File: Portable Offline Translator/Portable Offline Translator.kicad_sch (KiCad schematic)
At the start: 0 parts

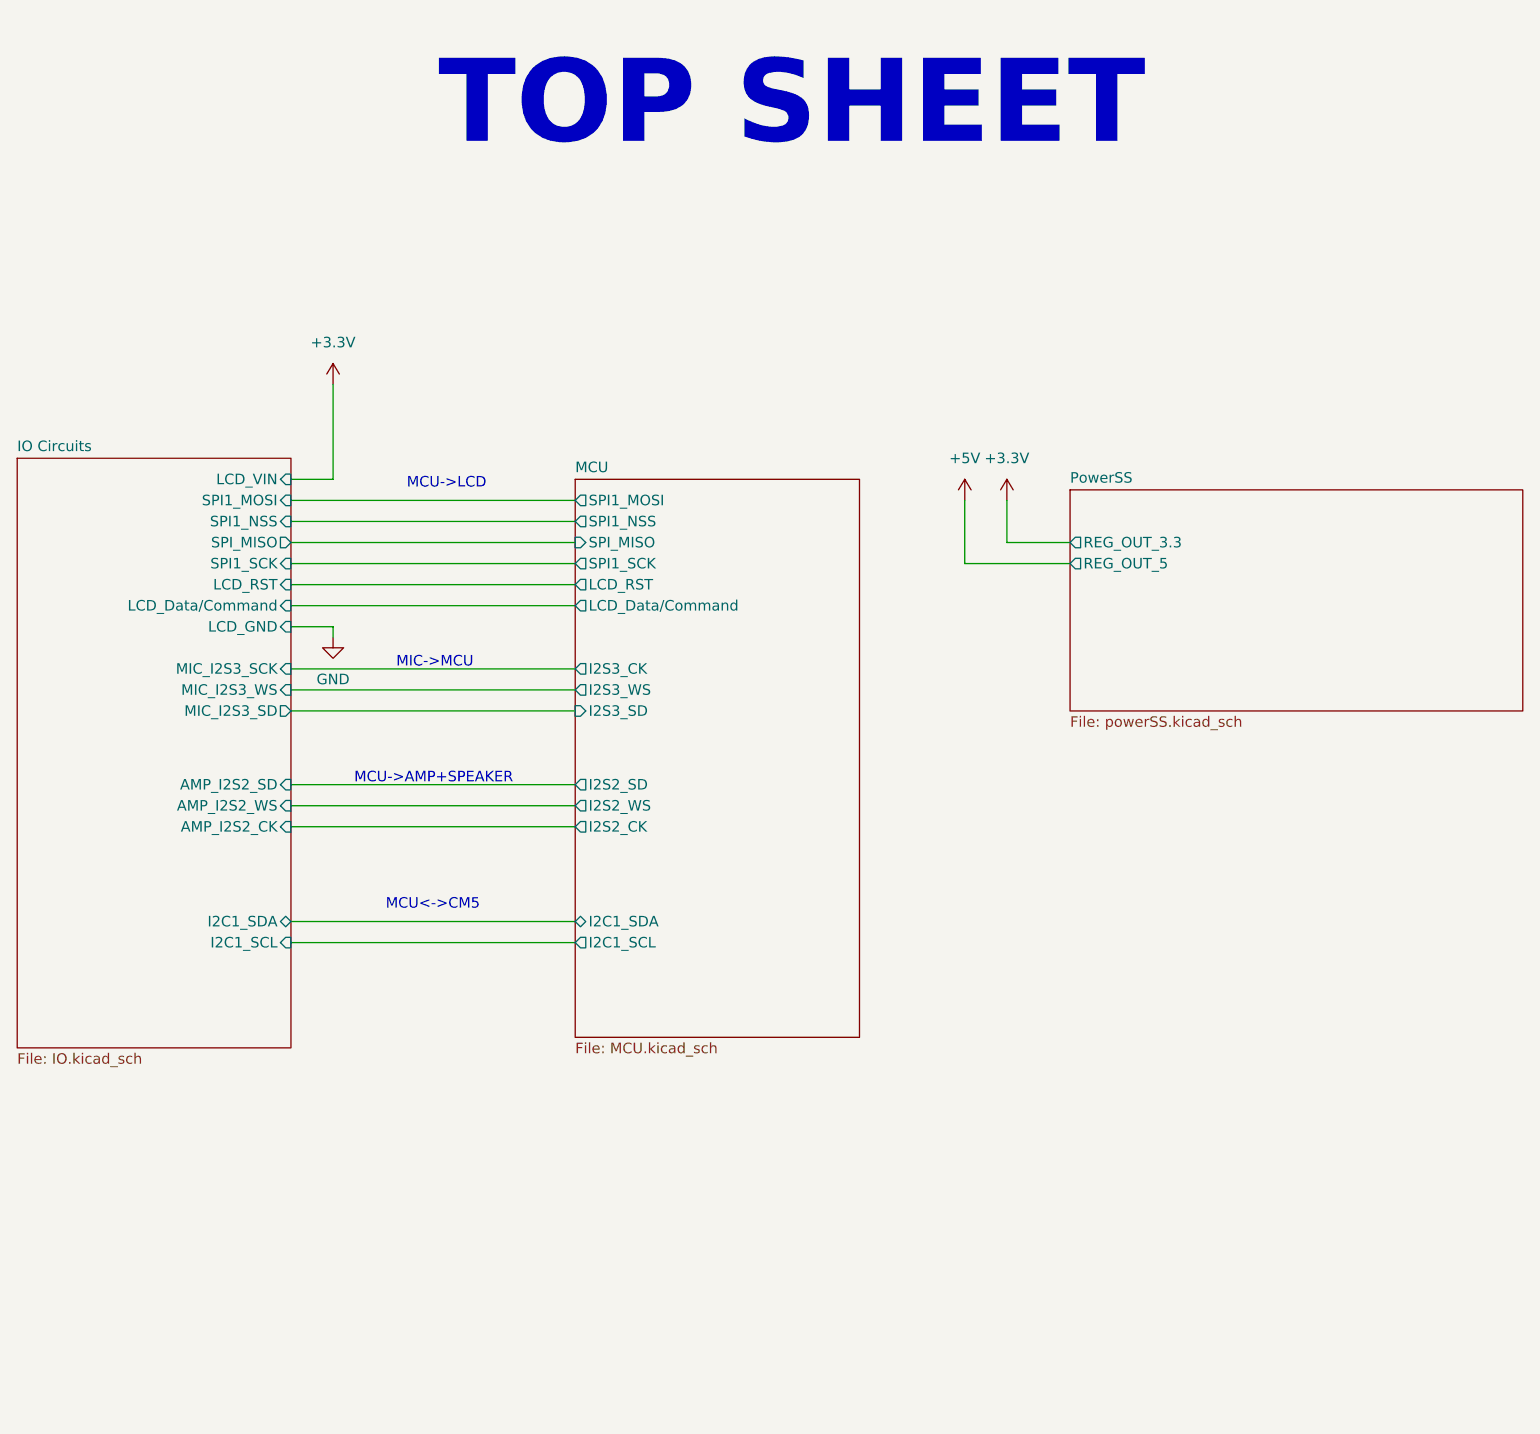
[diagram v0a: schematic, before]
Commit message: PCB iteration 1
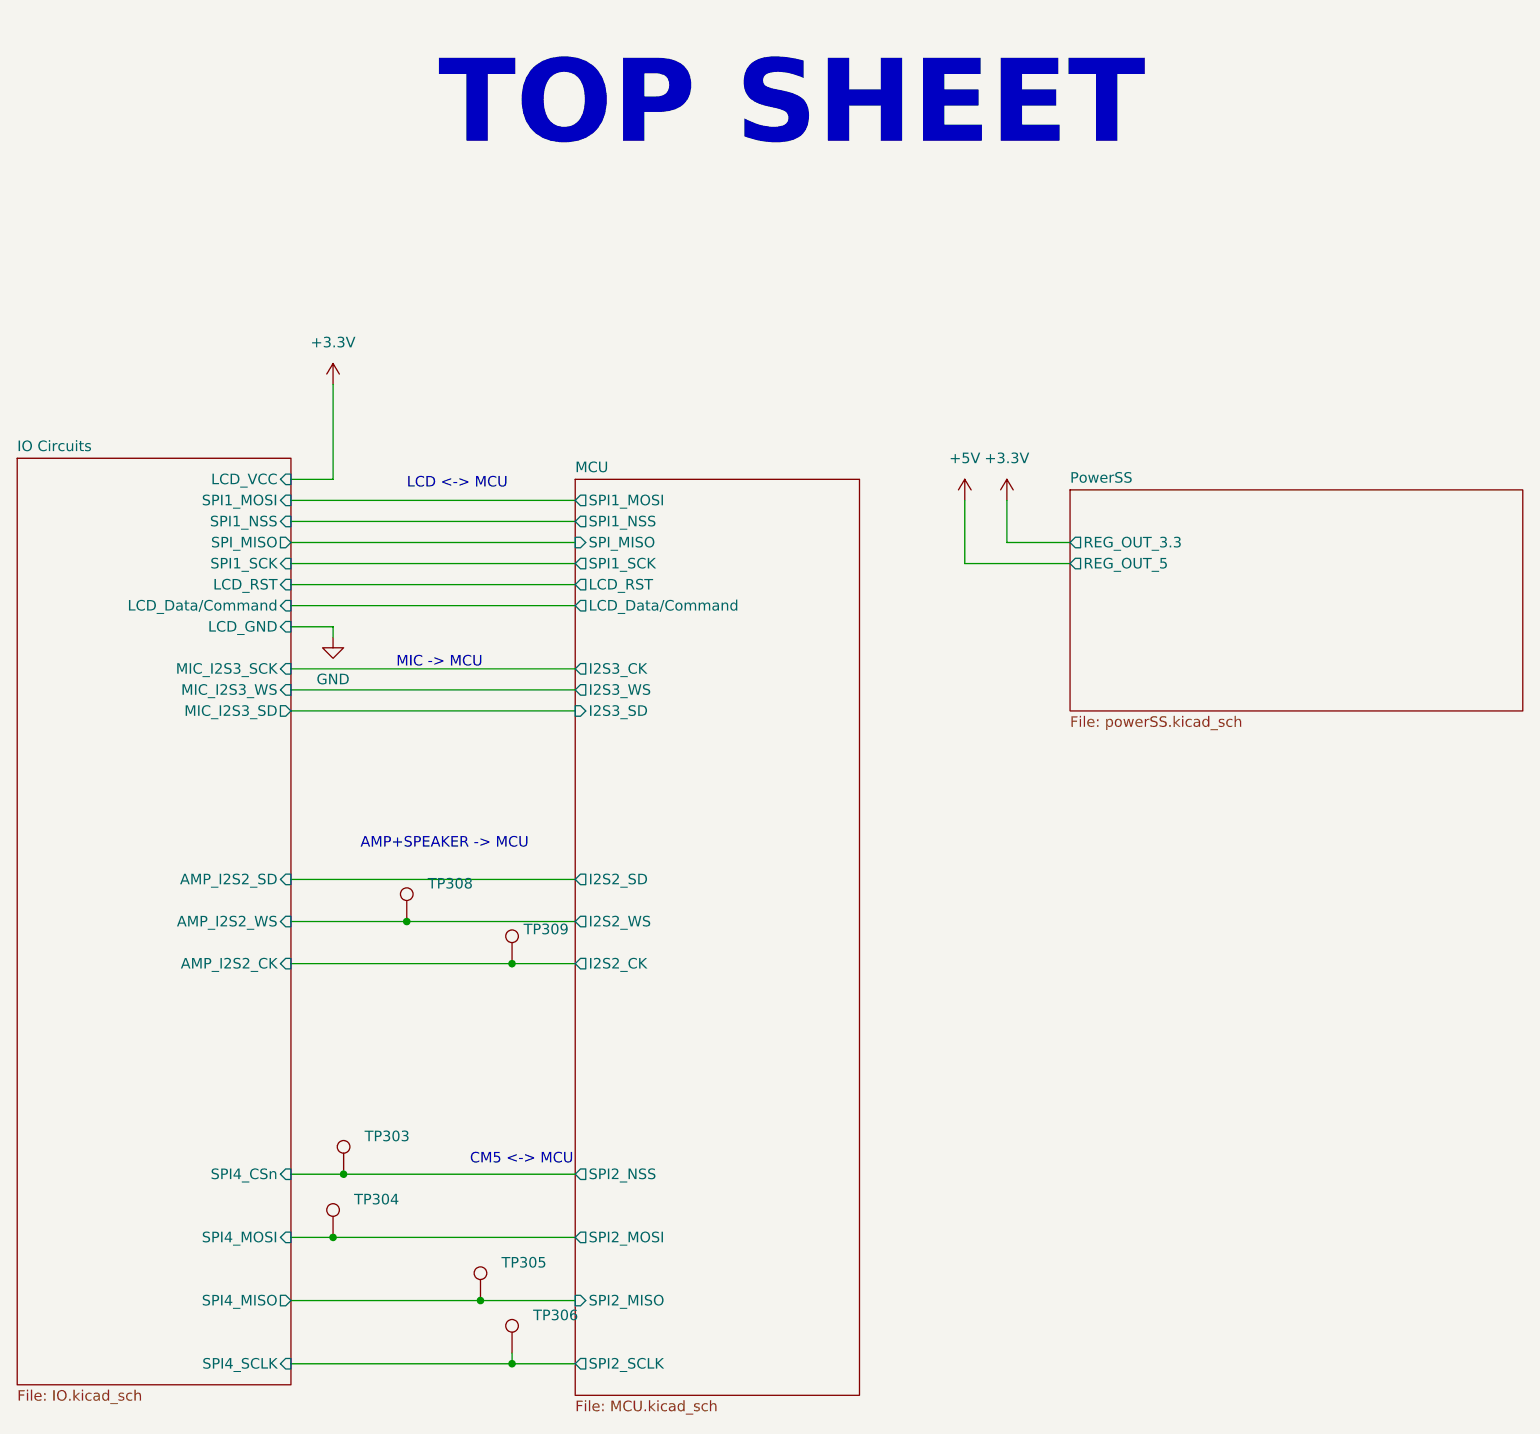
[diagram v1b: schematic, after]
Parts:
- added TP303: SPI4_CSn, TestPoint:TestPoint_Keystone_5000-5004_Miniature, symbol Connector:TestPoint
- added TP304: SPI4_MOSI, TestPoint:TestPoint_Keystone_5000-5004_Miniature, symbol Connector:TestPoint
- added TP305: SPI4_MISO, TestPoint:TestPoint_Keystone_5000-5004_Miniature, symbol Connector:TestPoint
- added TP306: SPI4_SCLK, TestPoint:TestPoint_Keystone_5000-5004_Miniature, symbol Connector:TestPoint
- added TP308: I2S_CLK, TestPoint:TestPoint_Keystone_5000-5004_Miniature, symbol Connector:TestPoint
- added TP309: 3.3V, TestPoint:TestPoint_Keystone_5000-5004_Miniature, symbol Connector:TestPoint
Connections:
- net IO Circuits/AMP_I2S2_CK: now also TP309.1
- net IO Circuits/AMP_I2S2_WS: now also TP308.1
- new net IO Circuits/SPI4_CSn: TP303.1
- new net IO Circuits/SPI4_MISO: TP305.1
- new net IO Circuits/SPI4_MOSI: TP304.1
- new net IO Circuits/SPI4_SCLK: TP306.1
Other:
- sheet IO Circuits ports: added LCD_VCC, SPI4_CSn, SPI4_MISO, SPI4_MOSI, SPI4_SCLK; removed I2C1_SCL, I2C1_SDA, LCD_VIN
- sheet MCU ports: added SPI2_MISO, SPI2_MOSI, SPI2_NSS, SPI2_SCLK; removed I2C1_SCL, I2C1_SDA
- note added: "AMP+SPEAKER -> MCU"
- note added: "CM5 <-> MCU"
- note added: "LCD <-> MCU"
- note added: "MIC -> MCU"
- note removed: "MCU->AMP+SPEAKER"
- note removed: "MCU->LCD"
- note removed: "MCU<->CM5"
- note removed: "MIC->MCU"
